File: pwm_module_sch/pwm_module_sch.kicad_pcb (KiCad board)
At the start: 2 copper layers, 55 parts, among them J1 SWIMM, J2 output -, J3 input, J4 output+, J5 uart, Q1 AO3400, Q2 IRFZ44N, SW1 ., SW2 ., U1 TM1637, U2 STM8S003F3P, U3 LM358, U4 L78L33

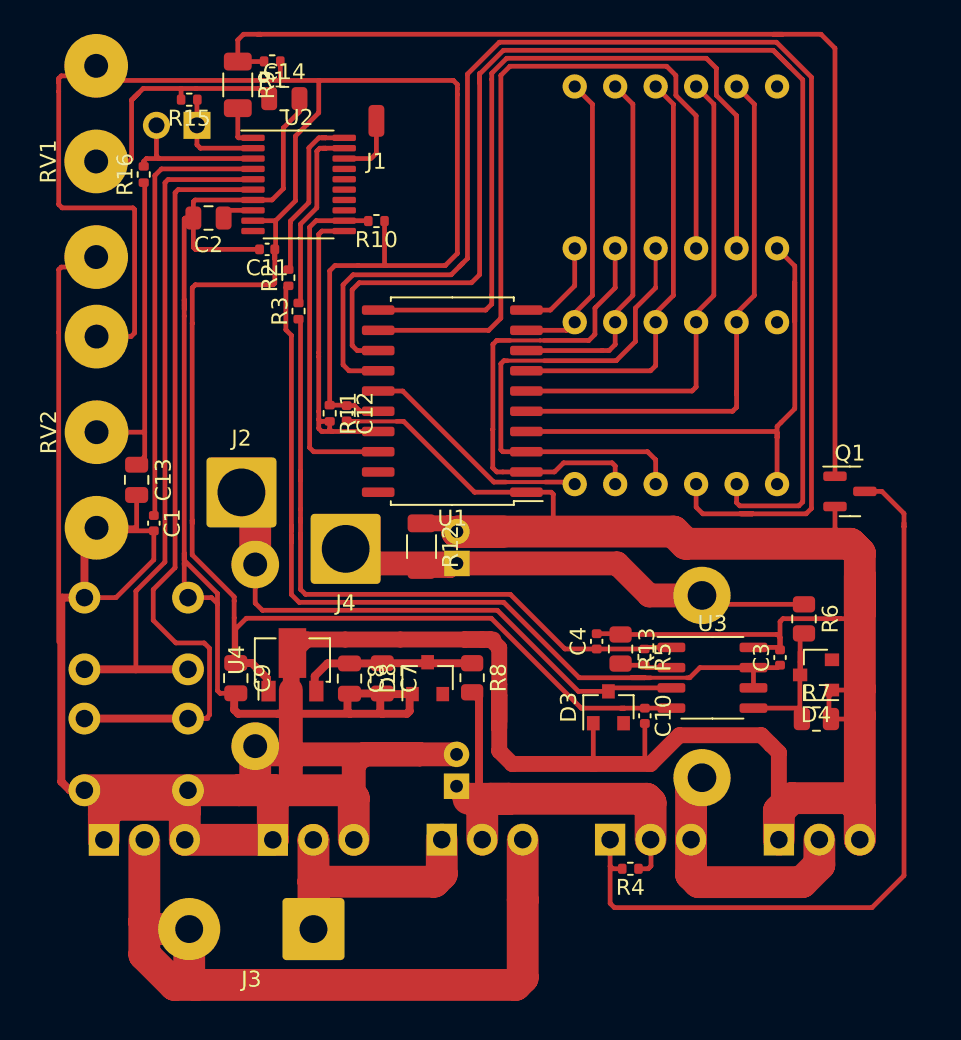
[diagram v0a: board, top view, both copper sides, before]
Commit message: board fixed
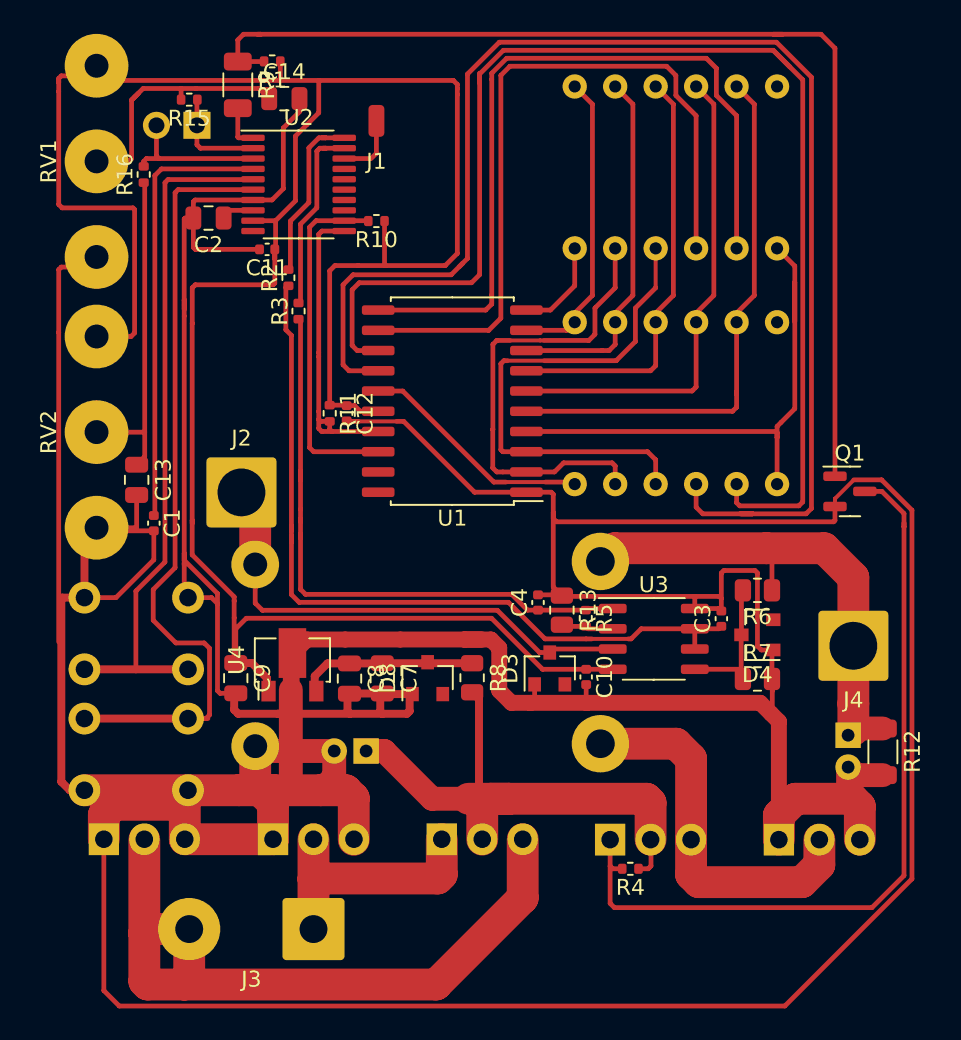
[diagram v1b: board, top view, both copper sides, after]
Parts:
- moved J4 32.4 mm to (233.8, 87.7)
- moved D5 31.8 mm to (229.2, 99.8)
- moved R12 31.7 mm to (235.7, 94.3), turned to 90 degrees
- moved C5 26.8 mm to (233.5, 93.3), turned to 270 degrees
- moved D7 21.2 mm to (186.8, 99.8)
- moved D9 21.2 mm to (208.0, 99.8)
- moved D6 10.6 mm to (197.4, 99.8)
- moved L1 6.72 mm to (218.0, 93.8)
- moved C6 6.09 mm to (203.3, 94.3), turned to 180 degrees
- moved R7 4.48 mm to (227.8, 89.8)
- moved D4 4.46 mm to (227.8, 87.0)
- moved U3 4.42 mm to (221.3, 87.2)
- moved C10 4.42 mm to (217.1, 89.6)
- moved C3 4.42 mm to (225.5, 86.0)
- moved C4 4.42 mm to (214.0, 85.0)
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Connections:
- D7 pad 1: Net-(D5-Pad2) -> GND
- D7 pad 2: +24V -> Net-(D7-Pad2)
- D7 pad 3: Net-(D6-Pad2) -> GND
- D9 pad 1: GND -> Net-(D6-Pad2)
- D9 pad 2: Net-(D9-Pad2) -> +24V
- D9 pad 3: GND -> Net-(D7-Pad2)
- J3 pad 1: Net-(D5-Pad2) -> Net-(D6-Pad2)
- J3 pad 2: Net-(D6-Pad2) -> Net-(D7-Pad2)
- L1 pad 1: Net-(D9-Pad2) -> Net-(D5-Pad2)
- Q2 pad 3: Net-(D9-Pad2) -> Net-(D5-Pad2)
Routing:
- net Net-(D7-Pad2): track 0.00 -> 45.2 mm
- net GND: track 378.7 -> 422.9 mm
- net Net-(D6-Pad2): track 47.3 -> 16.0 mm
- net Net-(D9-Pad2): track 16.6 -> 0.00 mm
- net Net-(D5-Pad2): track 16.0 -> 23.6 mm
- net +24V: track 28.9 -> 35.4 mm
- net Net-(C3-Pad1): track 55.5 -> 50.0 mm
- net +3V3: track 165.9 -> 161.0 mm
- net -VSW: track 37.4 -> 32.7 mm
- net Net-(C4-Pad1): track 42.8 -> 38.1 mm
- net Net-(D4-Pad1): track 10.1 -> 8.49 mm
